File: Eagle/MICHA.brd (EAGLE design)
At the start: 110.5 x 83.1 mm, 57 parts, among them IC1 LM4041A12LP, K1 PIN20X2, T1 BSS84, U1 ARDUINO_MKR_ZERO, U2 MIKROE_CLICK, X1 RJ45-RJULE4318101, X2 RJ45-RJULE4318101, X3 RJ45-RJULE4318101, X4 RJ45-RJULE4318101, X5 RJ45-RJULE4318101, X6 RJ45-RJULE4318101, X7 BUCHANAN_4_3.5MM

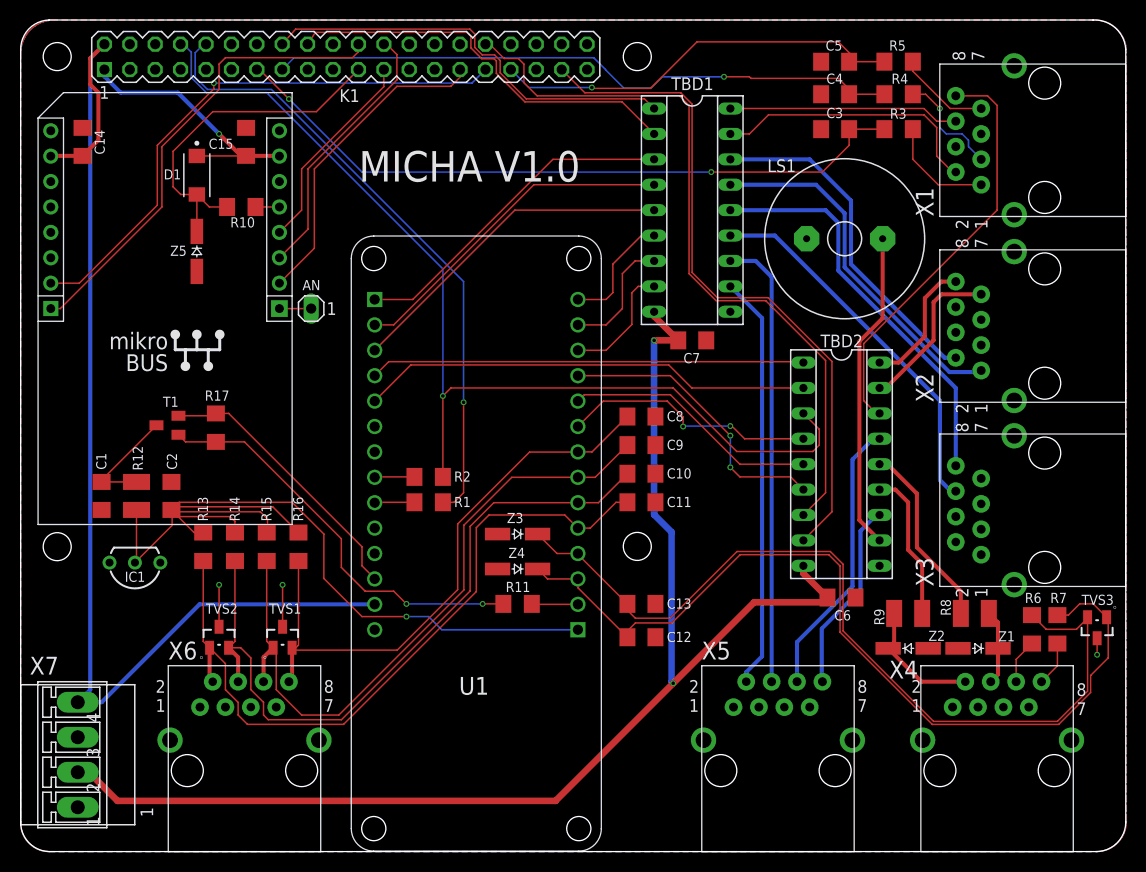
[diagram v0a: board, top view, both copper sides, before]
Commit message: Downgrade to current version of PCB
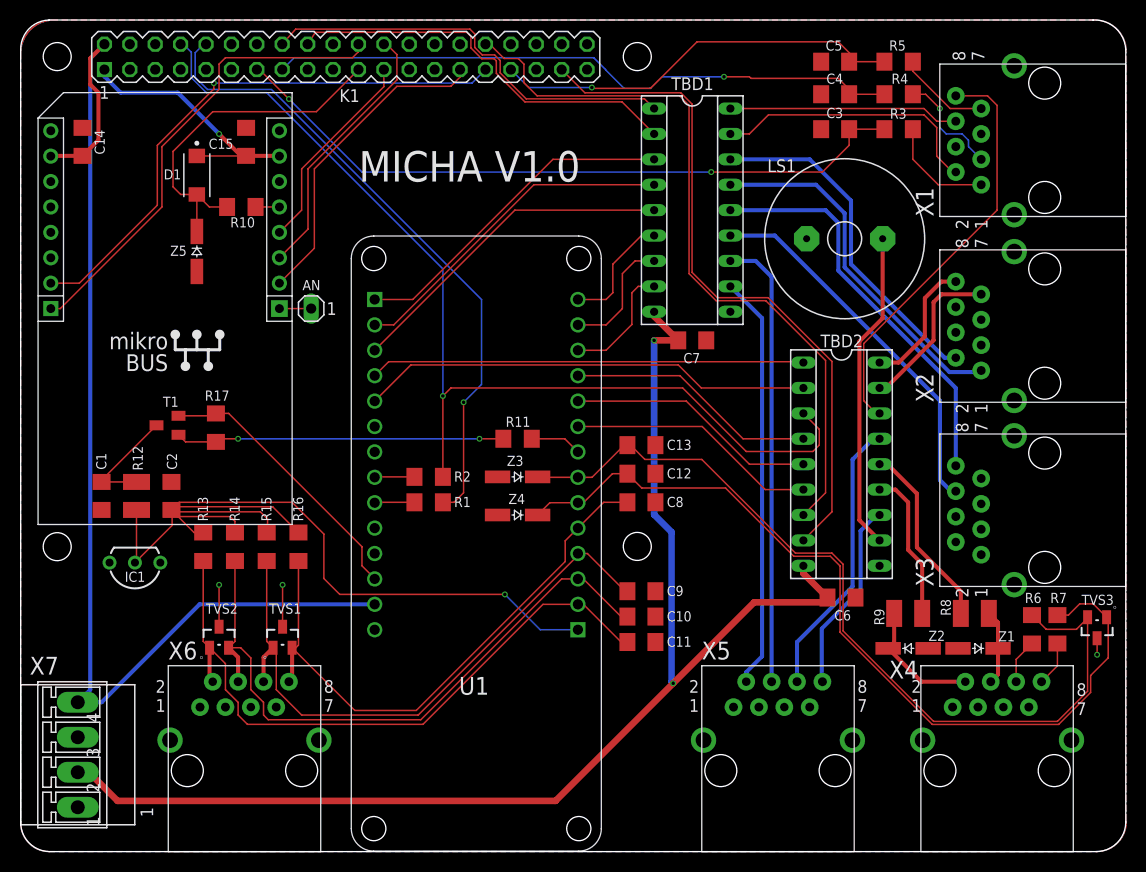
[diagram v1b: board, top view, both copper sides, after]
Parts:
- R6, R7: value 15-1/4W -> 2k
- Z1, Z2: value 5,1V-1W -> 5,1V/1W
- moved R11 16.5 mm to (49.5, 14.3)
- moved C12 16.4 mm to (61.9, 10.8)
- moved C13 15.9 mm to (61.9, 13.7)
- moved C9 14.6 mm to (61.9, -0.95)
- moved C10 14.3 mm to (61.9, -3.49)
- moved C11 14.0 mm to (61.9, -6.03)
- moved C8 8.57 mm to (61.9, 7.94)
- moved Z3 5.71 mm to (49.5, 10.5)
- moved Z4 5.40 mm to (49.5, 6.67)
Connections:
- net SOL_HOT renamed SOL_WARM
- net VALVE1_DIR renamed VALVE1_CLOSE
- net VALVE1_POWER renamed VALVE1_OPEN
- net VALVE2_DIR renamed VALVE2_CLOSE
- net VALVE2_POWER renamed VALVE2_OPEN
- net D0: now also TBD2.6; no longer TBD2.4
- net D19: now also U1.J4_6; no longer U1.J4_3
- net D2: now also TBD2.4; no longer TBD2.6
- net D21: now also U1.J4_8; no longer U1.J4_2
- net N$14: now also U1.J4_7; no longer U1.J4_4
- net THERMI1: now also U1.J4_2; no longer U1.J4_5
- net THERMI2: now also U1.J4_3; no longer U1.J4_6
- net THERMI3: now also U1.J4_4; no longer U1.J4_7
- net THERMI4: now also U1.J4_5; no longer U1.J4_8
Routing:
- net N$3: track 41.2 -> 32.9 mm
- net THERMI1: track 73.7 -> 66.2 mm
- net THERMI3: track 68.2 -> 61.6 mm
- net THERMI2: track 72.2 -> 65.6 mm
- net D2: track 29.1 -> 25.2 mm, vias 2 -> 0
- net D19: track 88.9 -> 87.2 mm
- net RX_PI: track 62.8 -> 64.3 mm
- net THERMI4: track 59.7 -> 58.5 mm
- net N$14: track 87.9 -> 86.9 mm
- net D0: track 25.7 -> 25.2 mm, vias 2 -> 0
- net D1: track 25.7 -> 25.2 mm
- net D21: track 4.63 -> 5.15 mm
